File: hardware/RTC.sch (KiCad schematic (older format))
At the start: 3 parts, among them U4 DS3231M

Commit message: Changed to pure-serial topology. Changed to beefier mcu.
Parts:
- BT1: footprint Connector_PinHeader_2.54mm:PinHeader_1x02_P2.54mm_Vertical -> custom:QJ1220-2SMT
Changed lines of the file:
@@
 F 0 "BT1" H 3668 2396 50  0000 L CNN
 F 1 "CR1220 3V" H 3668 2305 50  0000 L CNN
-F 2 "Connector_PinHeader_2.54mm:PinHeader_1x02_P2.54mm_Vertical" V 3550 2360 50  0001 C CNN
+F 2 "custom:QJ1220-2SMT" V 3550 2360 50  0001 C CNN
 F 3 "~" V 3550 2360 50  0001 C CNN
 	1    3550 2300

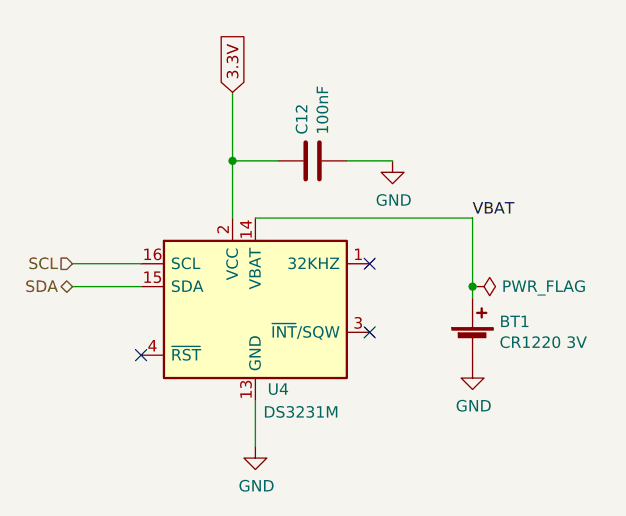
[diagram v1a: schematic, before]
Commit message: revE ready for production
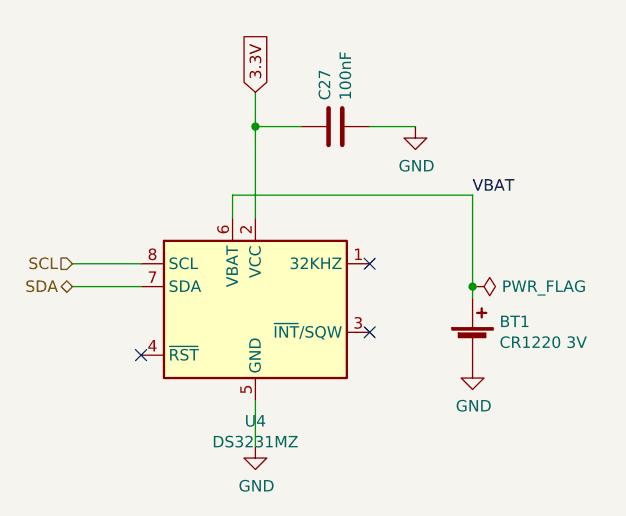
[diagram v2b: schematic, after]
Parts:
- removed U4: DS3231M, Package_SO:SOIC-16W_7.5x10.3mm_P1.27mm, symbol Timer_RTC:DS3231M
- added U4: DS3231MZ, Package_SO:SOIC-8_3.9x4.9mm_P1.27mm, symbol Timer_RTC:DS3231MZ
- BT1: footprint custom:QJ1220-2SMT -> custom:BatteryHolder_Linx_BAT-HLD-012-SMT
- renumbered C12 to C27
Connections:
- net 3.3V: now also U4.2 (VCC)
- net GND: now also U4.5 (GND)
- net SCL: now also U4.8 (SCL)
- net SDA: now also U4.7 (SDA)
- net VBAT: now also U4.6 (VBAT)
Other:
- moved on the sheet: C27
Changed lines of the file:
@@
-EESchema Schematic File Version 4
+EESchema Schematic File Version 5
 LIBS:pi-supercap-ups-cache
-EELAYER 26 0
+EELAYER 30 0
 EELAYER END
 $Descr A4 11693 8268
 encoding utf-8
-Sheet 5 8
+Sheet 7 7
 Title ""
 Date ""
@@
 Comment3 ""
 Comment4 ""
+Comment5 ""
+Comment6 ""
+Comment7 ""
+Comment8 ""
+Comment9 ""
 $EndDescr
 $Comp
-L Timer_RTC:DS3231M U4
-U 1 1 5C353AFF
-P 2600 2150
-F 0 "U4" H 2700 1800 50  0000 C CNN
-F 1 "DS3231M" H 2800 1700 50  0000 C CNN
-F 2 "Package_SO:SOIC-16W_7.5x10.3mm_P1.27mm" H 2600 1550 50  0001 C CNN
-F 3 "http://datasheets.maximintegrated.com/en/ds/DS3231.pdf" H 2870 2200 50  0001 C CNN
-	1    2600 2150
-	1    0    0    -1
-$EndComp
-$Comp
-L Device:C C12
+L Device:C C27
 U 1 1 5C353CB0
-P 2850 1500
-F 0 "C12" H 2965 1546 50  0000 L CNN
-F 1 "100nF" H 2965 1455 50  0000 L CNN
-F 2 "Capacitor_SMD:C_0603_1608Metric_Pad1.05x0.95mm_HandSolder" H 2888 1350 50  0001 C CNN
-F 3 "~" H 2850 1500 50  0001 C CNN
-	1    2850 1500
+P 2950 1350
+F 0 "C27" H 3065 1396 50  0000 L CNN
+F 1 "100nF" H 3065 1305 50  0000 L CNN
+F 2 "Capacitor_SMD:C_0603_1608Metric_Pad1.05x0.95mm_HandSolder" H 2988 1200 50  0001 C CNN
+F 3 "~" H 2950 1350 50  0001 C CNN
+	1    2950 1350
 	0    -1   -1   0
 $EndComp
-Text GLabel 2500 1200 1    50   Input ~ 0
+Text GLabel 2600 1200 1    50   Input ~ 0
 3.3V
 $Comp
 L power:GND #PWR035
 U 1 1 5C354469
-P 3200 1500
-F 0 "#PWR035" H 3200 1250 50  0001 C CNN
-F 1 "GND" H 3205 1327 50  0000 C CNN
-F 2 "" H 3200 1500 50  0001 C CNN
-F 3 "" H 3200 1500 50  0001 C CNN
-	1    3200 1500
+P 3300 1350
+F 0 "#PWR035" H 3300 1100 50  0001 C CNN
+F 1 "GND" H 3305 1177 50  0000 C CNN
+F 2 "" H 3300 1350 50  0001 C CNN
+F 3 "" H 3300 1350 50  0001 C CNN
+	1    3300 1350
 	1    0    0    -1
 $EndComp
@@
 F 0 "BT1" H 3668 2396 50  0000 L CNN
 F 1 "CR1220 3V" H 3668 2305 50  0000 L CNN
-F 2 "custom:QJ1220-2SMT" V 3550 2360 50  0001 C CNN
+F 2 "custom:BatteryHolder_Linx_BAT-HLD-012-SMT" V 3550 2360 50  0001 C CNN
 F 3 "~" V 3550 2360 50  0001 C CNN
 	1    3550 2300
@@
 $EndComp
 Wire Wire Line
-	2600 1750 3550 1750
+	2500 1650 3550 1650
 Wire Wire Line
-	3550 1750 3550 2050
+	3550 1650 3550 2050
 NoConn ~ 2100 2350
 NoConn ~ 3100 2250
@@
 	3550 2050 3550 2100
 Wire Wire Line
-	2500 1200 2500 1500
+	2600 1200 2600 1350
 Wire Wire Line
-	3200 1500 3000 1500
+	3300 1350 3100 1350
 Wire Wire Line
-	2700 1500 2500 1500
-Connection ~ 2500 1500
+	2800 1350 2600 1350
+Connection ~ 2600 1350
 Wire Wire Line
-	2500 1500 2500 1750
-Text Label 3550 1750 0    50   ~ 0
+	2600 1350 2600 1750
+Text Label 3550 1650 0    50   ~ 0
 VBAT
+$Comp
+L Timer_RTC:DS3231MZ U4
+U 1 1 5D77B733
+P 2600 2150
+F 0 "U4" H 2600 1661 50  0000 C CNN
+F 1 "DS3231MZ" H 2600 1570 50  0000 C CNN
+F 2 "Package_SO:SOIC-8_3.9x4.9mm_P1.27mm" H 2600 1650 50  0001 C CNN
+F 3 "http://datasheets.maximintegrated.com/en/ds/DS3231M.pdf" H 2600 1550 50  0001 C CNN
+	1    2600 2150
+	1    0    0    -1
+$EndComp
+Wire Wire Line
+	2500 1650 2500 1750
 $EndSCHEMATC
